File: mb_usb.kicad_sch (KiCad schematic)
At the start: 51 parts, among them J11 USB_A_Stacked, J8 USB_A_Stacked, J9 USB_C_Receptacle_USB2.0, U7 USB3320, U8 TPS2051BDBV, U9 GL850G, Y1 24Mhz, Y2 12Mhz

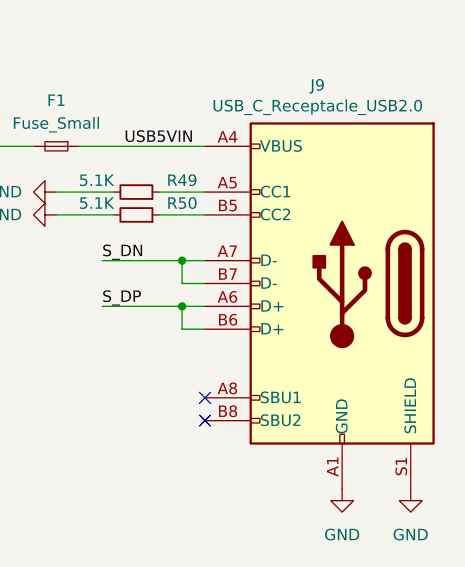
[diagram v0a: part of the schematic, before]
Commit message: finall version
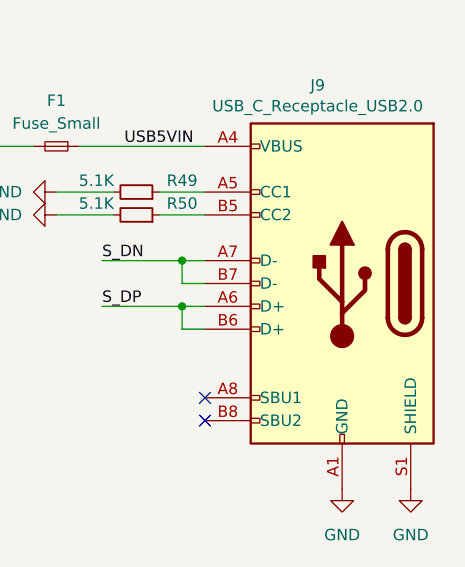
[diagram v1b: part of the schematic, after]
